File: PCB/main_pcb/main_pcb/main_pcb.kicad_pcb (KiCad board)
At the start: 2 copper layers, 235 x 235 mm, 49 parts, among them J1 Conn_01x20_Socket, J10 B6B-XH-A, J11 B8B-XH-A, J12 B6B-XH-A, J13 B8B-XH-A, J14 B8B-XH-A, J2 Conn_01x20_Socket, J3 B02P-VL, J4 B02P-VL, J5 B8B-XH-A, J6 B8B-XH-A, J7 B8B-XH-A, J8 B8B-XH-A, J9 B6B-XH-A, U1 MCP3208, U10 APDS-9006-020, U11 APDS-9006-020, U12 APDS-9006-020, U2 MCP3208, U3 APDS-9006-020, U4 APDS-9006-020, U5 APDS-9006-020, U6 APDS-9006-020, U7 APDS-9006-020, U8 APDS-9006-020, U9 APDS-9006-020

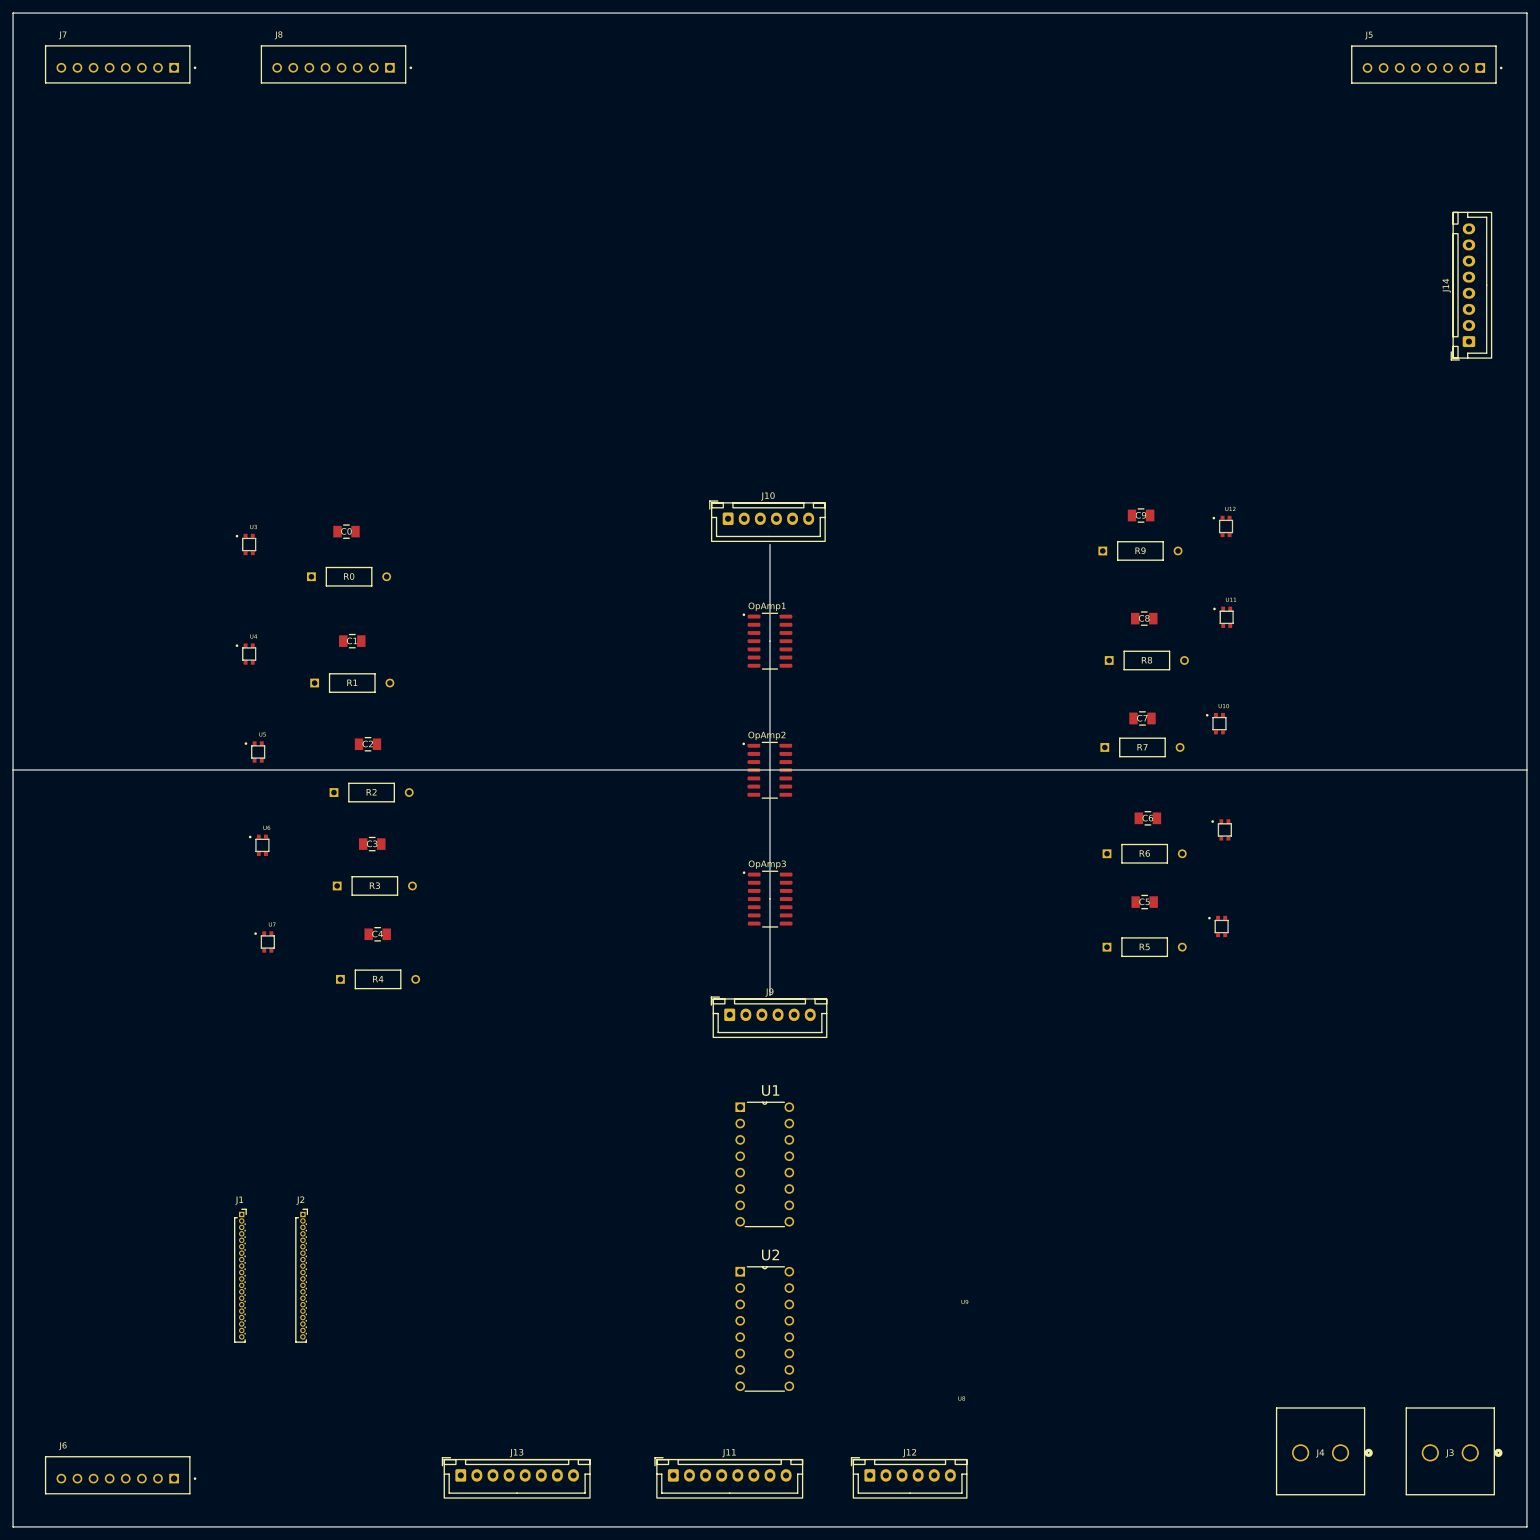
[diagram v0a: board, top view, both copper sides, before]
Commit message: Started layout of the main PCB. God help me for I have sinned :(
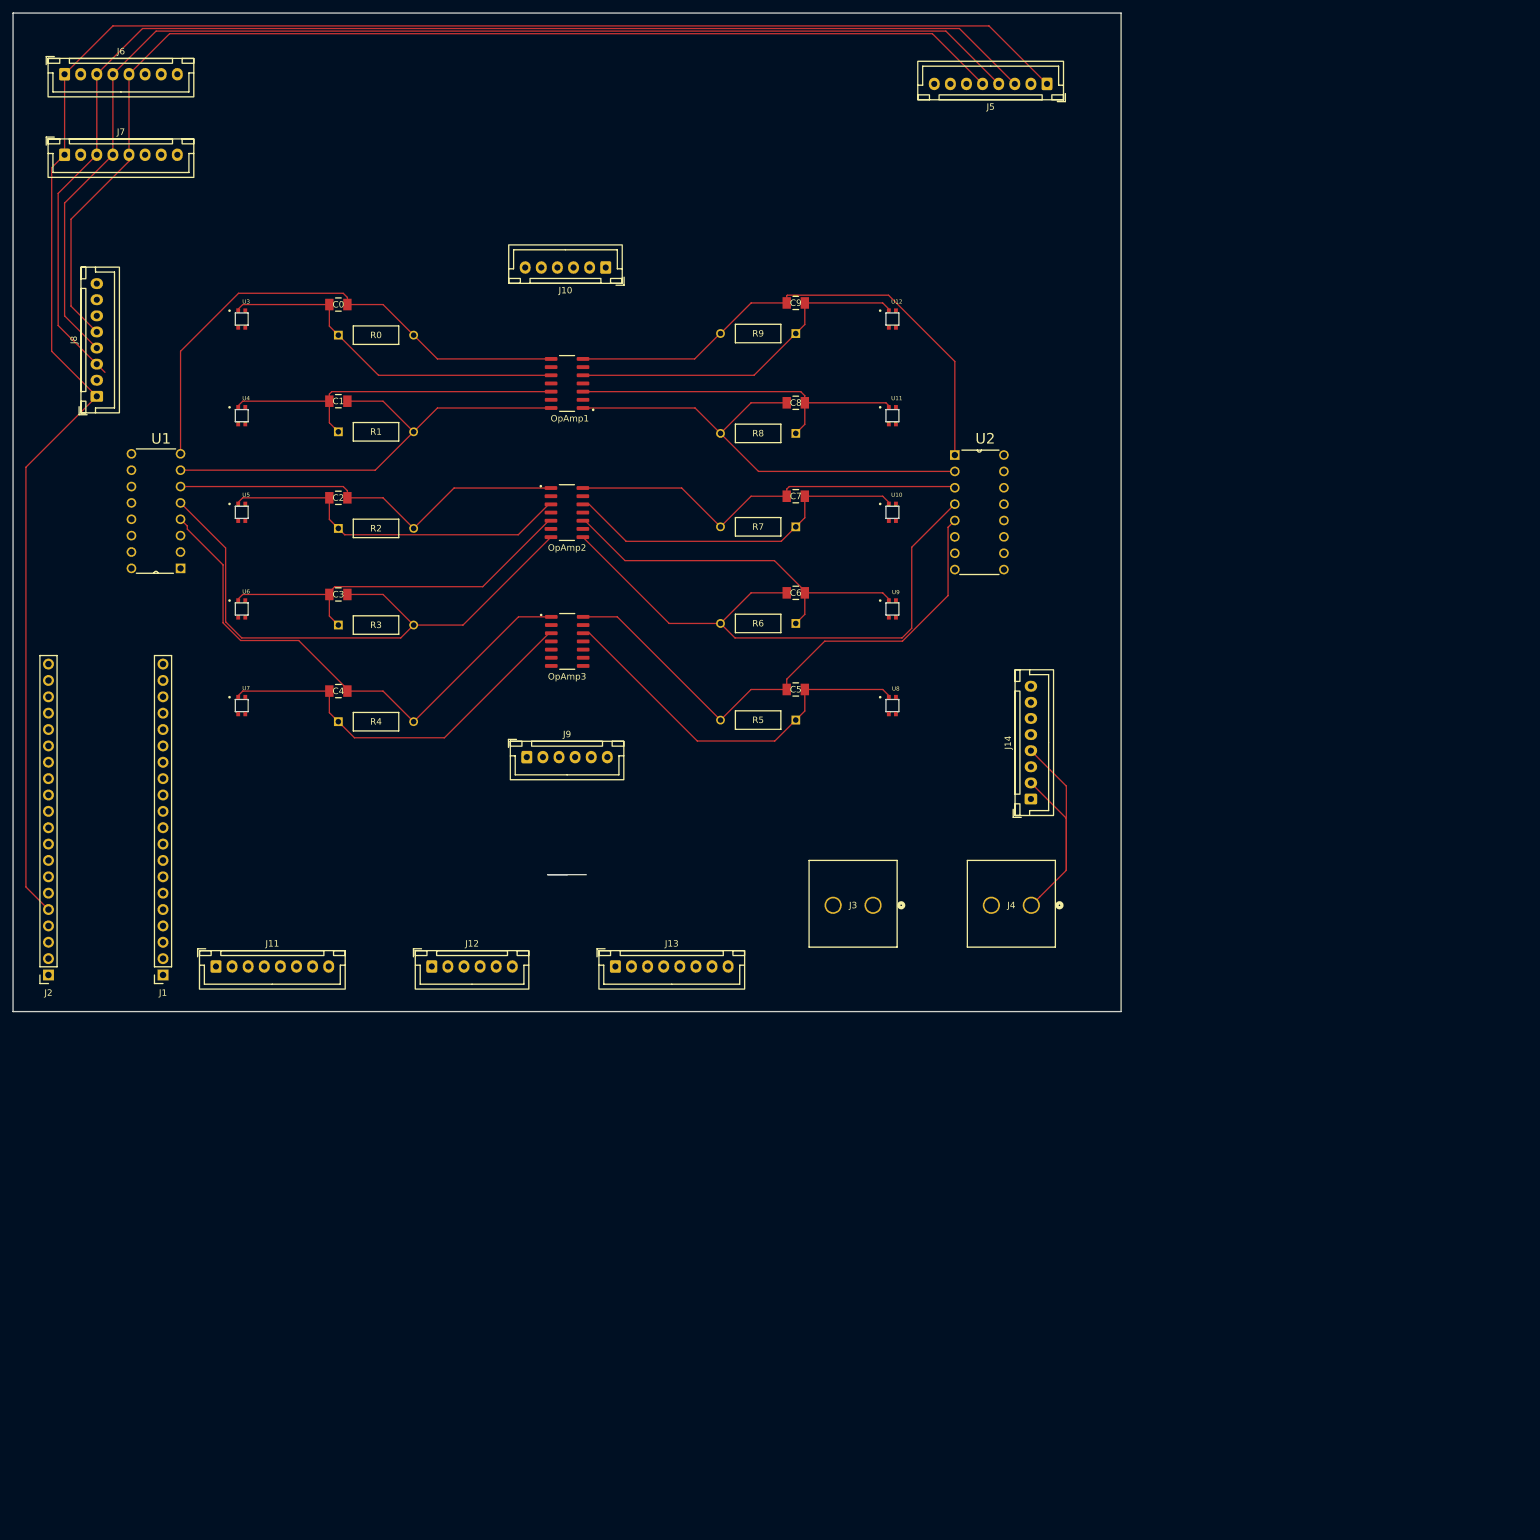
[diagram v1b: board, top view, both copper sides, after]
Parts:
- J1, J2: footprint Connector_PinSocket_1.00mm:PinSocket_1x20_P1.00mm_Vertical -> Connector_PinSocket_2.54mm:PinSocket_1x20_P2.54mm_Vertical
- J5, J6, J7, J8: footprint B8B_XH_A:JST_B8B-XH-A -> Connector_JST:JST_XH_B8B-XH-A_1x08_P2.50mm_Vertical
- moved J6 217.6 mm to (23.0, 24.5)
- moved U1 157.0 mm to (33.4, 83.4), turned to 180 degrees
- moved U2 131.1 mm to (168.8, 101.4)
- moved J3 125.8 mm to (148.5, 153.5)
- moved J11 106.2 mm to (46.5, 163.0)
- moved J12 104.2 mm to (80.0, 163.0)
- moved J14 98.3 mm to (173.0, 137.0)
- moved J4 97.6 mm to (173.1, 153.5)
- moved J13 82.6 mm to (108.5, 163.0)
- moved C6 64.9 mm to (136.5, 105.0), turned to 180 degrees
- moved C7 63.9 mm to (136.5, 90.0), turned to 180 degrees
- moved C8 63.6 mm to (136.5, 75.5), turned to 180 degrees
- moved C5 63.4 mm to (136.5, 120.0), turned to 180 degrees
- moved J8 63.3 mm to (28.0, 74.5), turned to 90 degrees
- moved C9 62.9 mm to (136.5, 60.0), turned to 180 degrees
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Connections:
- C2 pad 1: OpIn2 -> OpIn4
- C2 pad 2: OpOut2 -> OpOut4
- C3 pad 1: OpIn3 -> OpIn5
- C3 pad 2: OpOut3 -> OpOut5
- C4 pad 1: OpIn4 -> OpIn8
- C4 pad 2: OpOut4 -> OpOut8
- C5 pad 1: OpIn5 -> OpIn9
- C5 pad 2: OpOut5 -> OpOut9
- C6 pad 1: OpIn6 -> OpIn7
- C6 pad 2: OpOut6 -> OpOut7
- C7 pad 1: OpIn7 -> OpIn6
- C7 pad 2: OpOut7 -> OpOut6
- C8 pad 1: OpIn8 -> OpIn3
- C8 pad 2: OpOut8 -> OpOut3
- C9 pad 1: OpIn9 -> OpIn2
- C9 pad 2: OpOut9 -> OpOut2
- J1 pad 2: SPI1_CDn_SD -> unconnected-(J1-Pin_2-Pad2)
- J13 pad 4: SPI1_TX -> GND
- J13 pad 5: SPI1_RX -> SPI1_TX
- J13 pad 6: SPI1_CSn_SD -> SPI1_RX
- J13 pad 7: SPI1_CDn_SD -> SPI1_CSn_SD
- J13 pad 8: unconnected-(J13-Pad8) -> GND
- J3 pad 2: GND -> HEATER_ON
- OpAmp1 pad 1: OpOut0 -> OpOut3
- OpAmp1 pad 10: OpIn2 -> OpIn0
- OpAmp1 pad 12: OpIn3 -> OpIn1
- OpAmp1 pad 14: OpOut3 -> OpOut1
- OpAmp1 pad 3: OpIn0 -> OpIn3
- OpAmp1 pad 5: OpIn1 -> OpIn2
- OpAmp1 pad 7: OpOut1 -> OpOut2
- OpAmp1 pad 8: OpOut2 -> OpOut0
- OpAmp2 pad 10: OpIn6 -> OpIn7
- OpAmp2 pad 12: OpIn7 -> OpIn6
- OpAmp2 pad 14: OpOut7 -> OpOut6
- OpAmp2 pad 8: OpOut6 -> OpOut7
- OpAmp3 pad 12: unconnected-(OpAmp3-IN4+-Pad12) -> OpIn9
- OpAmp3 pad 14: unconnected-(OpAmp3-OUT4-Pad14) -> OpOut9
- OpAmp3 pad 5: OpIn9 -> unconnected-(OpAmp3-IN2+-Pad5)
- OpAmp3 pad 7: OpOut9 -> unconnected-(OpAmp3-OUT2-Pad7)
- R2 pad 1: OpIn2 -> OpIn4
- R2 pad 2: OpOut2 -> OpOut4
- R3 pad 1: OpIn3 -> OpIn5
- R3 pad 2: OpOut3 -> OpOut5
- R4 pad 1: OpIn4 -> OpIn8
- R4 pad 2: OpOut4 -> OpOut8
- R5 pad 1: OpIn5 -> OpIn9
- R5 pad 2: OpOut5 -> OpOut9
- R6 pad 1: OpIn6 -> OpIn7
- R6 pad 2: OpOut6 -> OpOut7
- R7 pad 1: OpIn7 -> OpIn6
- R7 pad 2: OpOut7 -> OpOut6
- R8 pad 1: OpIn8 -> OpIn3
- R8 pad 2: OpOut8 -> OpOut3
- R9 pad 1: OpIn9 -> OpIn2
- R9 pad 2: OpOut9 -> OpOut2
- U1 pad 1: OpOut5 -> unconnected-(U1-CH0-Pad1)
- U1 pad 2: OpOut6 -> unconnected-(U1-CH1-Pad2)
- U1 pad 3: OpOut7 -> unconnected-(U1-CH2-Pad3)
- U1 pad 5: OpOut9 -> OpOut5
- U1 pad 6: unconnected-(U1-CH5-Pad6) -> OpOut4
- U1 pad 7: unconnected-(U1-CH6-Pad7) -> OpOut1
- U1 pad 8: unconnected-(U1-CH7-Pad8) -> OpOut0
- U10 pad 1: OpIn7 -> OpIn6
- U11 pad 1: OpIn8 -> OpIn3
- U12 pad 1: OpIn9 -> OpIn2
- U2 pad 1: OpOut0 -> OpOut2
- U2 pad 2: OpOut1 -> OpOut3
- U2 pad 3: OpOut2 -> OpOut6
- U2 pad 4: OpOut3 -> OpOut7
- U2 pad 5: OpOut4 -> OpOut9
- U4 pad 1: OpIn1 -> unconnected-(U4-OUT-Pad1)
- U4 pad 2: +3.3V -> unconnected-(U4-VCC-Pad2)
- U4 pad 3: +3.3V -> unconnected-(U4-VCC__1-Pad3)
- U5 pad 1: OpIn2 -> OpIn4
- U6 pad 1: OpIn3 -> OpIn5
- U7 pad 1: OpIn4 -> OpIn8
- U8 pad 1: OpIn5 -> OpIn9
- U9 pad 1: OpIn6 -> OpIn7
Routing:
- net +3.3V: track 0.00 -> 298.7 mm
- net I2C0_SCL: track 0.00 -> 200.8 mm
- net I2C0_SDA: track 0.00 -> 191.3 mm
- net TEMP_ALERT: track 0.00 -> 183.7 mm
- net OpOut7: track 0.00 -> 92.4 mm
- net OpOut5: track 0.00 -> 91.6 mm
- net OpOut9: track 0.00 -> 84.3 mm
- net OpOut8: track 0.00 -> 83.0 mm
- net OpOut0: track 0.00 -> 82.4 mm
- net OpOut2: track 0.00 -> 81.2 mm
- net OpOut1: track 0.00 -> 74.8 mm
- net OpOut3: track 0.00 -> 74.6 mm
- net OpOut6: track 0.00 -> 63.5 mm
- net OpOut4: track 0.00 -> 63.4 mm
- net OpIn8: track 0.00 -> 60.6 mm
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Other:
- board size 235 x 235 mm -> 172 x 155 mm
